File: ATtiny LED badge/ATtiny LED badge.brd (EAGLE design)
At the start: 50.8 x 50.8 mm, 29 parts

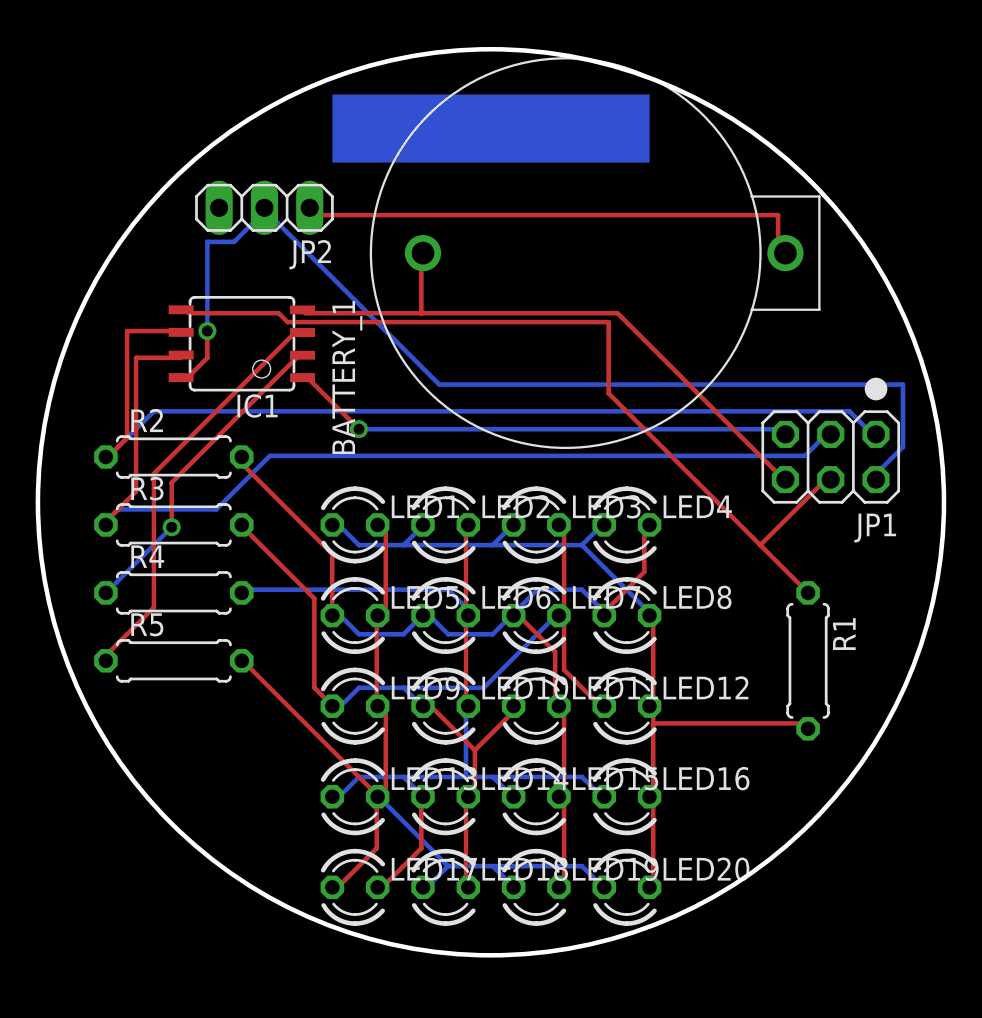
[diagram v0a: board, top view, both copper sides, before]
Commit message: routed PCBs
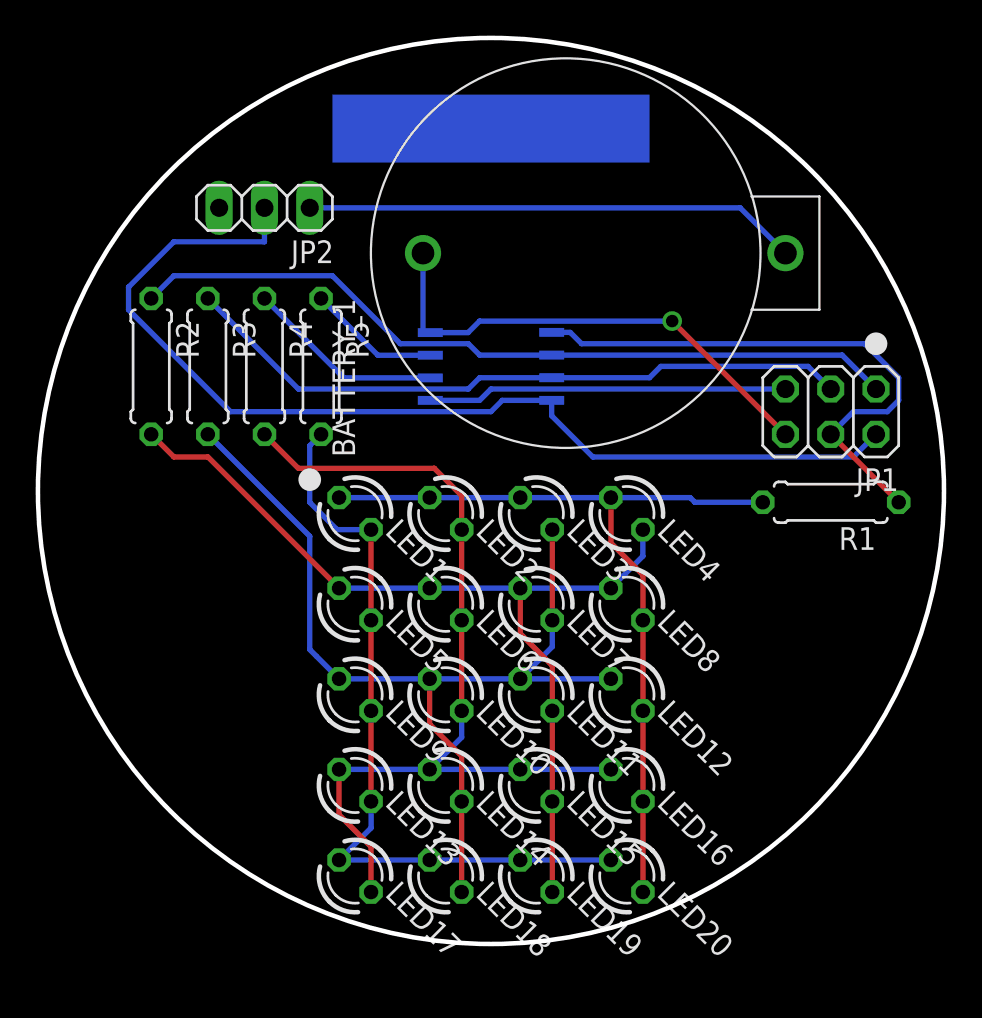
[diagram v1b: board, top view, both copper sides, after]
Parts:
- moved R5 18.5 mm to (15.9, 33.0), turned to 270 degrees
- moved IC1 14.0 mm to (25.4, 33.0), flipped to the bottom
- moved R4 13.7 mm to (12.7, 33.0), turned to 270 degrees
- moved R3 9.09 mm to (9.53, 33.0), turned to 270 degrees
- moved R1 8.98 mm to (44.5, 25.4), turned to 180 degrees
- moved R2 5.24 mm to (6.35, 33.0), turned to 270 degrees
- moved JP1 2.54 mm to (44.5, 30.5)
- moved LED1 0.64 mm to (17.8, 24.8), turned to 315 degrees
- moved LED2 0.64 mm to (22.9, 24.8), turned to 315 degrees
- moved LED3 0.64 mm to (27.9, 24.8), turned to 315 degrees
- moved LED4 0.64 mm to (33.0, 24.8), turned to 315 degrees
- moved LED17 0.64 mm to (17.8, 4.45), turned to 315 degrees
- moved LED18 0.64 mm to (22.9, 4.45), turned to 315 degrees
- moved LED19 0.64 mm to (27.9, 4.45), turned to 315 degrees
- moved LED20 0.64 mm to (33.0, 4.45), turned to 315 degrees
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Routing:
- net MOSI: track 49.5 -> 31.8 mm
- net SCK: track 55.5 -> 38.1 mm
- net PB4: track 23.2 -> 7.44 mm
- net MISO: track 55.4 -> 43.8 mm
- net N$5: track 51.7 -> 42.7 mm
- net RST: track 28.4 -> 20.2 mm, vias 1 -> 0
- net PB3: track 18.0 -> 11.1 mm, vias 1 -> 0
- net GND: track 34.4 -> 27.7 mm, vias 0 -> 1
- net N$1: track 49.6 -> 46.7 mm
- net N$4: track 53.5 -> 51.4 mm
- net N$3: track 55.6 -> 53.8 mm
- net N$2: track 52.4 -> 51.2 mm
- net N$6: track 28.9 -> 27.7 mm
- net VCC: track 58.4 -> 58.7 mm, vias 1 -> 0
